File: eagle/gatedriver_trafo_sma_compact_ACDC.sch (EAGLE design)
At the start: 43 parts, among them K1 G5V-2, X4 BU-SMA-V

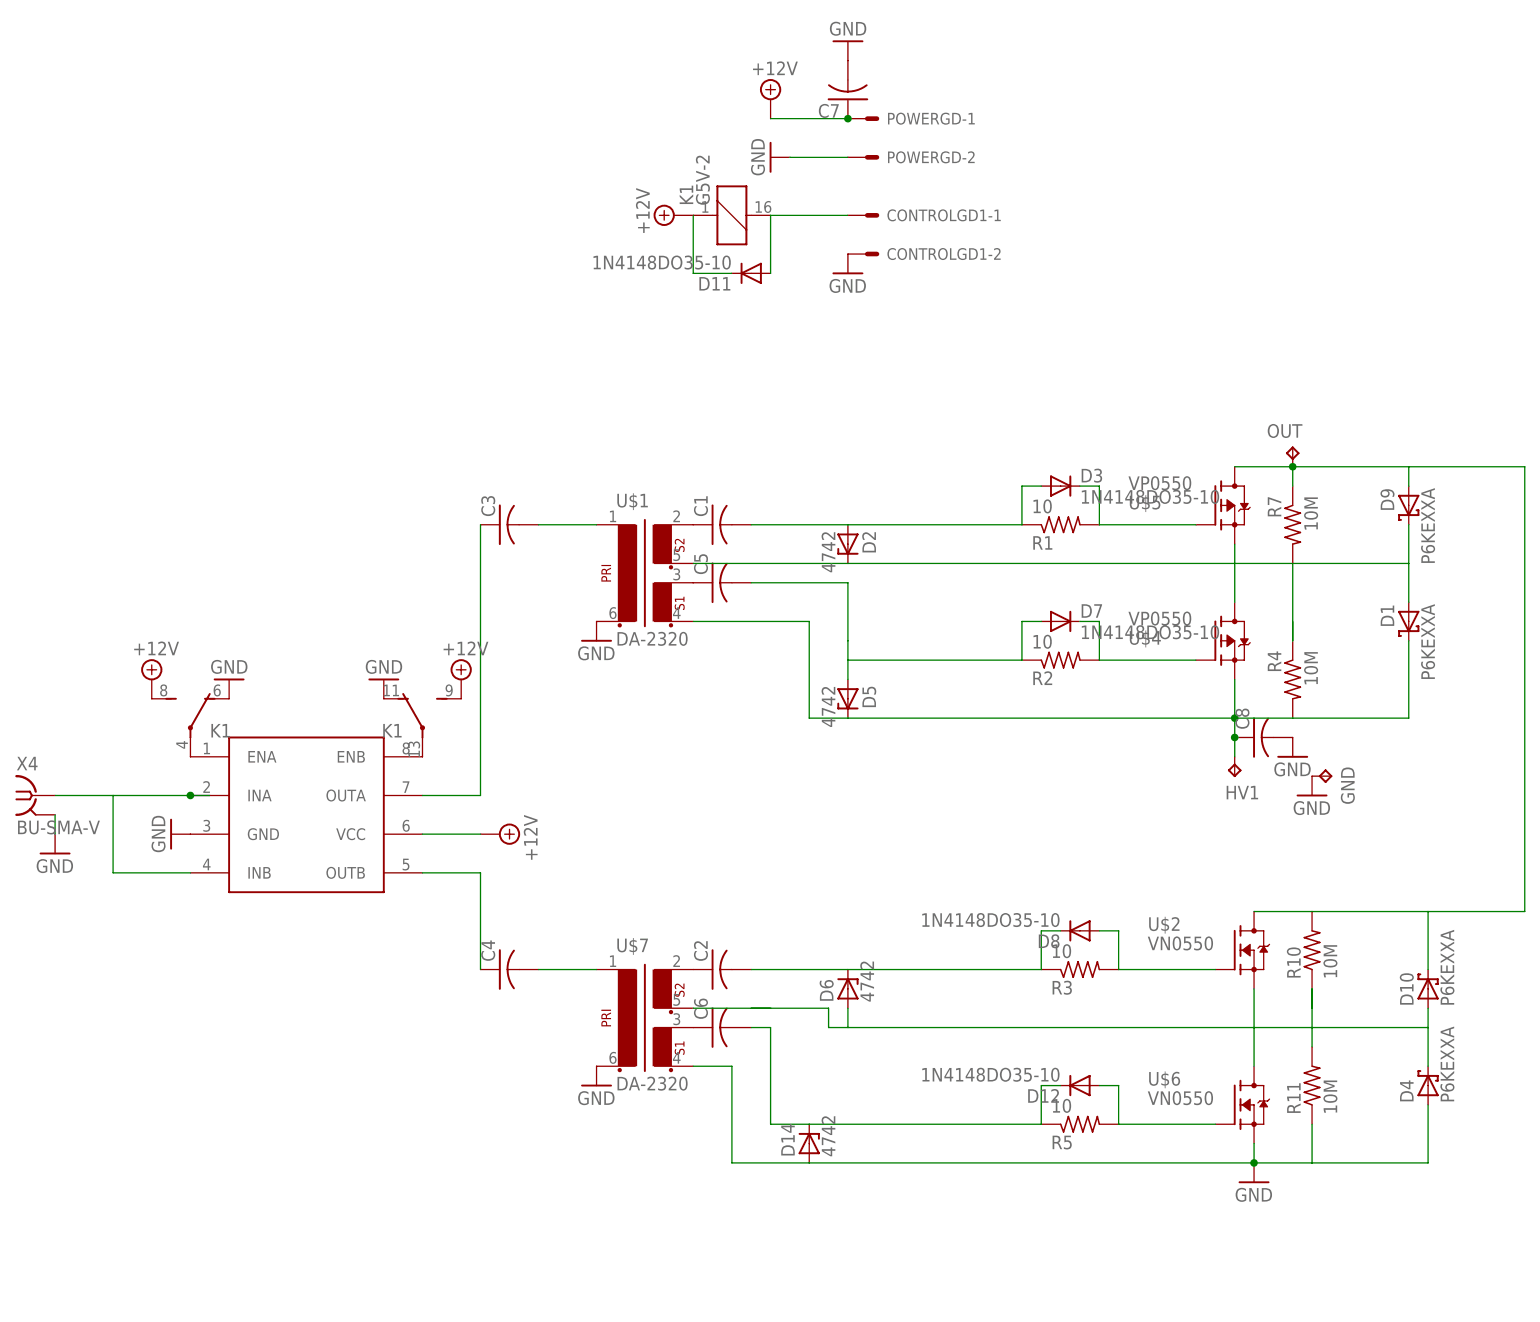
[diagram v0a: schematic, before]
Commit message: IXYS board solution, gatedriver components
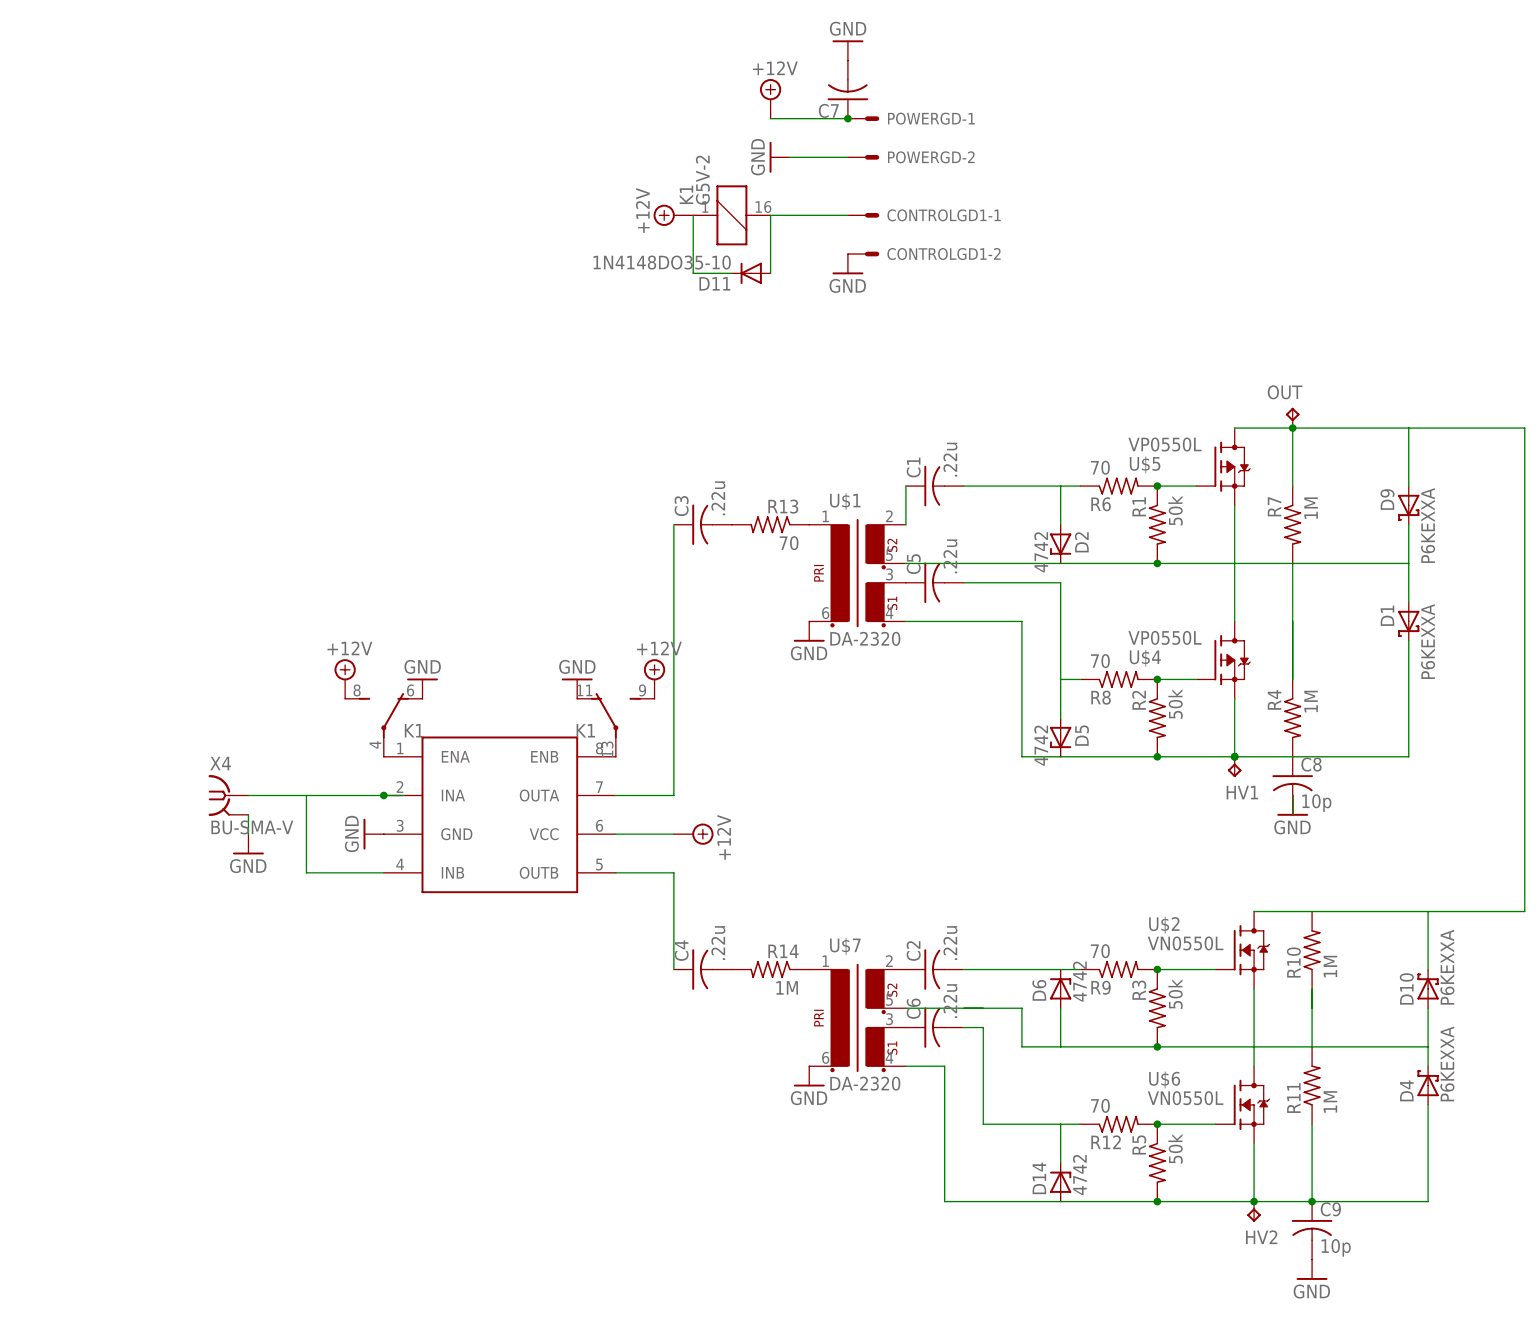
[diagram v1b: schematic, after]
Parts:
- removed D12, D3, D7, D8: 1N4148DO35-10, diode:1N4148DO35-10
- removed GND: TPPAD1-20Y, testpad:TPPAD1-20Y
- added C9: 10p, resistor:C-US102-064X133
- added HV2: TPPAD1-20Y, testpad:TPPAD1-20Y
- added R12, R13, R6, R8, R9: 70, rcl:R-US_0207/10
- added R14: 1M, rcl:R-US_0207/10
- C1, C2, C3, C4, C5, C6: value (none) -> .22u
- C8: value (none) -> 10p; device rcl:C-US102-054X133 -> resistor:C-US102-064X133
- R1, R2, R3, R5: value 10 -> 50k; device rcl:R-US_0207/12 -> rcl:R-US_0207/10
- R10, R11, R4, R7: value 10M -> 1M; device rcl:R-US_0207/12 -> rcl:R-US_0207/10
- U$2, U$6: value VN0550 -> VN0550L; device transistor-fet:VN0550 -> transistor-fet:VN0550L
- U$4, U$5: value VP0550 -> VP0550L; device transistor-fet:VP0550 -> transistor-fet:VP0550L
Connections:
- new net N$16: C5.2, D5.A, R8.1
- new net N$20: C4.2, R14.2
- new net N$251: R3.1, R9.2, U$2.G
- net GND: now also C9.2; no longer D14.A, D4.A, GND.TP, R11.1, U$6.S, U$7.3
- net N$10: now also R6.1; no longer D3.A, R1.1
- net N$11: now also R12.2, R5.1, U$6.G; no longer D7.C, R2.2, U$4.G
- net N$12: now also R8.2, U$4.G; no longer C5.2, D5.A, D7.A
- net N$13: now also R3.2
- net N$17: now also R2.2
- net N$18: now also R1.2
- net N$19: now also C3.2, R13.2; no longer D8.A, R3.2, U$2.G
- net N$24: now also C9.1, D14.A, D4.A, HV2.TP, R11.1, U$6.S, U$7.3; no longer D12.A, U$6.G
- net N$25: now also R9.1; no longer D8.C, R3.1
- net N$27: now also R12.1; no longer D12.C, R5.1
- net N$3: now also R13.1; no longer C3.2
- net N$6: now also R14.1; no longer C4.2
- net N$8: now also R1.1, R6.2; no longer D3.C, R1.2
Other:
- moved on the sheet: C1, C2, C3, C4, C5, C6, C8, D14, D2, D5, D6, K1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
